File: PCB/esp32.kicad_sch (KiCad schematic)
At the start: 8 parts, among them J2 E-Ink Connector, SW1 B1, SW2 B2, SW3 B3, SW4 B4, U4 DS3231 Breakout, U5 MicroSD Breakout, U6 ESP-WROOM-32 Dev Module

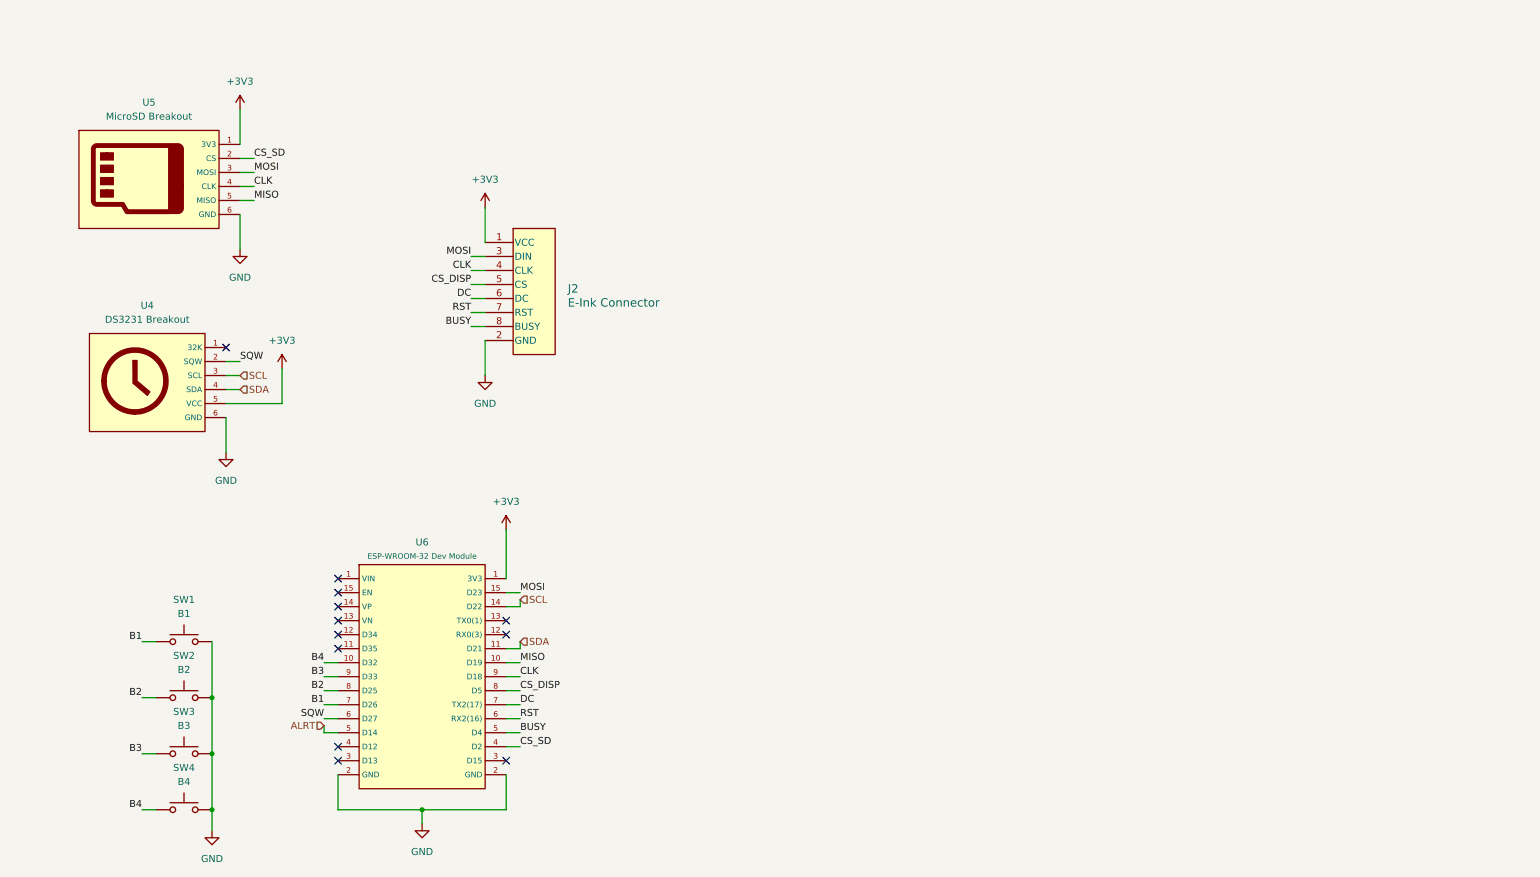
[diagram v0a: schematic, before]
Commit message: PCB Routing
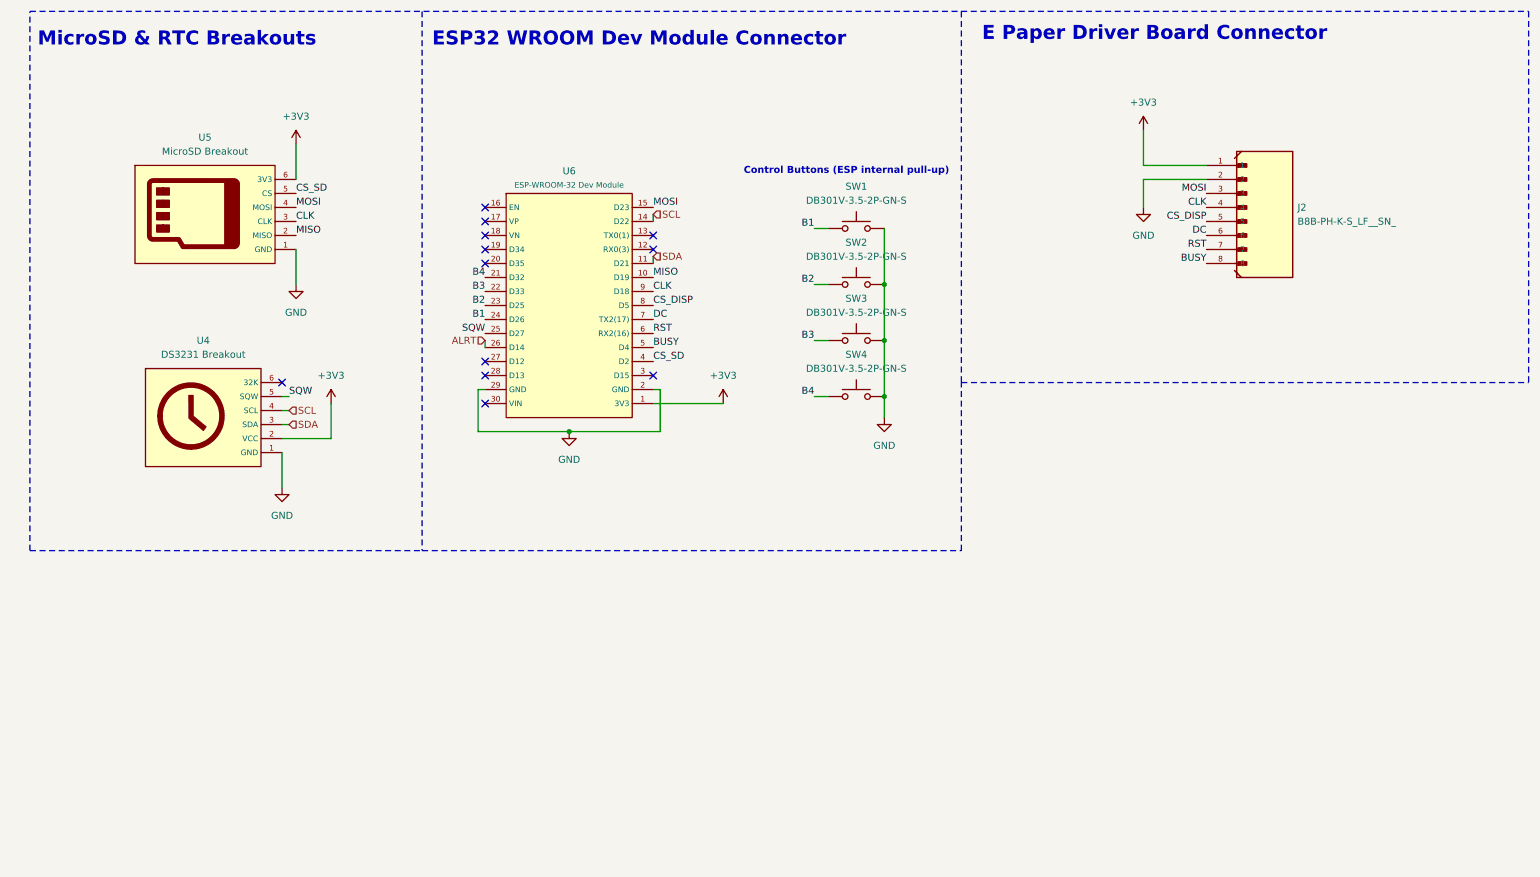
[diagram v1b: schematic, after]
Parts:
- removed J2: E-Ink Connector, CONN_BM08B-SRSS-TBLFSN_JST, symbol BM08B_SRSS_TB:BM08B-SRSS-TBLFSN
- added J2: B8B-PH-K-S_LF__SN_, B8B-PH-K-S_LF__SN_:JST_B8B-PH-K-S_LF__SN_, symbol B8B-PH-K-S_LF__SN_:B8B-PH-K-S_LF__SN_
- SW1: value B1 -> DB301V-3.5-2P-GN-S; footprint (none) -> 1984617:PHOENIX_1984617
- SW2: value B2 -> DB301V-3.5-2P-GN-S; footprint (none) -> 1984617:PHOENIX_1984617
- SW3: value B3 -> DB301V-3.5-2P-GN-S; footprint (none) -> 1984617:PHOENIX_1984617
- SW4: value B4 -> DB301V-3.5-2P-GN-S; footprint (none) -> 1984617:PHOENIX_1984617
- U4, U5: footprint (none) -> Connector_PinSocket_2.54mm:PinSocket_1x06_P2.54mm_Vertical
- U6: footprint (none) -> ESP32-DEVKIT-V1:MODULE_ESP32_DEVKIT_V1
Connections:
- net +3V3: now also U4.2 (VCC), U5.6 (3V3), J2.1; no longer U4.5 (VCC), U5.1 (3V3)
- net ALRT: now also U6.26 (D14); no longer U6.5 (D4)
- net B1: now also U6.24 (D26); no longer U6.7 (TX2(17))
- net B2: now also U6.23 (D25); no longer U6.8 (D5)
- net B3: now also U6.22 (D33); no longer U6.9 (D33)
- net B4: now also U6.21 (D32); no longer U6.10 (D32)
- net BUSY: now also J2.8
- net CLK: now also U5.3 (CLK), J2.4; no longer U5.4 (CLK)
- net CS_DISP: now also J2.5
- net CS_SD: now also U5.5 (CS); no longer U5.2 (CS)
- net DC: now also J2.6
- net GND: now also U4.1 (GND), U5.1 (GND), U6.29 (GND), J2.2; no longer U4.6 (GND), U5.6 (GND)
- net MISO: now also U5.2 (MISO); no longer U5.5 (MISO)
- net MOSI: now also U5.4 (MOSI), J2.3; no longer U5.3 (MOSI)
- net RST: now also J2.7
- net SCL: now also U4.4 (SCL); no longer U4.3 (SCL)
- net SDA: now also U4.3 (SDA); no longer U4.4 (SDA)
- net SQW: now also U4.5 (SQW), U6.25 (D27); no longer U4.2 (SQW), U6.6 (RX2(16))
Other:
- note added: "Control Buttons (ESP internal pull-up)"
- note added: "E Paper Driver Board Connector"
- note added: "ESP32 WROOM Dev Module Connector"
- note added: "MicroSD & RTC Breakouts"
- moved on the sheet: SW1, SW2, SW3, SW4, U4, U5, U6
